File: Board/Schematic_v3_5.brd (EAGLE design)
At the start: 100 x 80 mm, 34 parts, among them IC1 MCP73831T-2ACI_OT, IC2 LP38692MP-3.3_NOPB, IC3 ESP32-S3-WROOM-1-N16R8, IC4 AD8226ARZ, IC5 LMV321IDBVRE4, IC6 LMV321IDBVRE4, J1 USB3500-30-A-KIT, J2 SJ-3523-SMT-TR, J3 1769

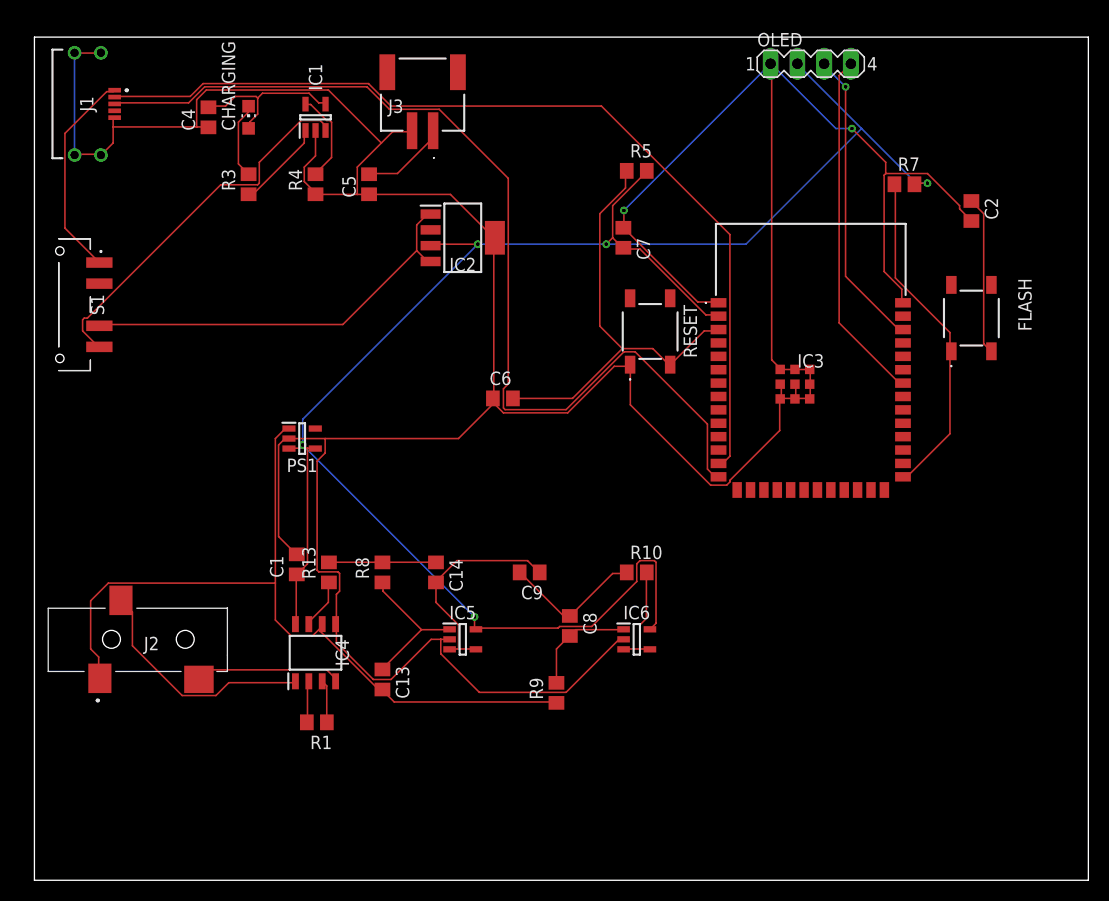
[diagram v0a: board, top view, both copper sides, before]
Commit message: Primer diseño de la pcb
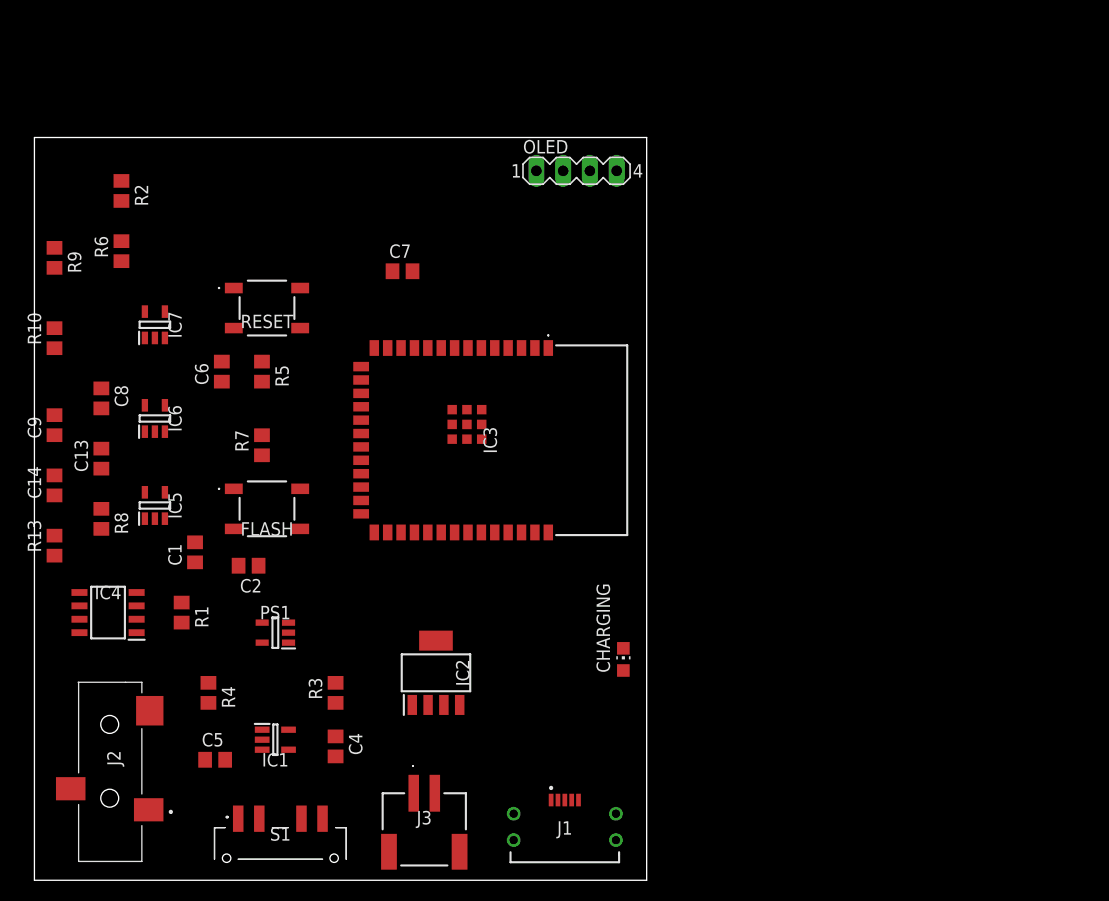
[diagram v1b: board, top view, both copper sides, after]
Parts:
- added IC7: LMV321IDBVRE4, LMV321IDBVRE4:SOT95P280X145-5N
- added R2, R6: (no value), rcl:R0805
- moved J1 83.9 mm to (50.3, 3.81), turned to 0 degrees
- moved C2 76.4 mm to (20.3, 29.8), turned to 180 degrees
- moved FLASH 69.2 mm to (22.1, 35.2), turned to 0 degrees
- moved R7 65.8 mm to (21.6, 41.3), turned to 90 degrees
- moved R9 63.0 mm to (1.91, 59.1), turned to 270 degrees
- moved J3 62.9 mm to (37.0, 8.26), turned to 0 degrees
- moved CHARGING 62.5 mm to (55.9, 21.0)
- moved C4 60.9 mm to (28.6, 12.7), turned to 270 degrees
- moved R10 59.5 mm to (1.91, 51.4), turned to 90 degrees
- moved IC1 59.2 mm to (22.9, 13.3), turned to 0 degrees
- moved C5 56.5 mm to (17.1, 11.4), turned to 0 degrees
- moved S1 54.7 mm to (23.3, 3.49), turned to 0 degrees
- moved IC6 50.3 mm to (11.4, 43.8), turned to 90 degrees
- moved C8 49.4 mm to (6.35, 45.7)
- moved R4 49.3 mm to (16.5, 17.8), turned to 270 degrees
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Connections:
- removed net OUT_ADC: IC3.7
- new net VOUT4: IC3.7, IC7.4, R6.1
- net +3V3: now also IC7.5
- net +BATT: now also C5.2, J3.1, S1.B1; no longer S1.D1
- net GND: now also IC7.2
- net N$14: now also IC7.3, R2.2, R6.2; no longer C5.2, J3.1
- net VOUT3: now also IC7.1
- net VSS: now also R2.1
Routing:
- net GND: track 347.6 -> 0.00 mm, vias 2 -> 0
- net +3V3: track 183.3 -> 0.00 mm, vias 5 -> 0
- net +D: track 93.8 -> 0.00 mm
- net -D: track 87.3 -> 0.00 mm
- net VSS: track 76.2 -> 0.00 mm
- net RESET32: track 42.3 -> 0.00 mm
- net N$13: track 39.0 -> 0.00 mm
- net +BATT: track 36.0 -> 0.00 mm
- net SDA: track 33.5 -> 0.00 mm
- net N$10: track 32.2 -> 0.00 mm
- net SCL: track 28.6 -> 0.00 mm, vias 1 -> 0
- net N$3: track 22.8 -> 0.00 mm
- net VOUT2: track 20.9 -> 0.00 mm
- net +5V: track 20.0 -> 0.00 mm
- net N$15: track 15.5 -> 0.00 mm
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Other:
- board size 100 x 80 mm -> 58.1 x 70.5 mm
